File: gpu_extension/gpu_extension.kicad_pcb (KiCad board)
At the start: 4 copper layers, 70 x 50 mm, 89 parts, among them J1 Conn_02x10_Odd_Even, J2 DB15_Female_HighDensity_Mount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, J201 Conn_01x03_Male, J202 Conn_01x03_Male, J302 NOT_HDMI_A, Q1 BS170F, Q2 BS170F, Q3 BS170F, Q4 BS170F, U1 W25Q32JVSS, U2 IPS1604, U4 RP2040, U403 W25Q128JVS, U6 RP2040, Y201 ECS-120-8-36-CGN-TR, Y202 ECS-120-8-36-CGN-TR

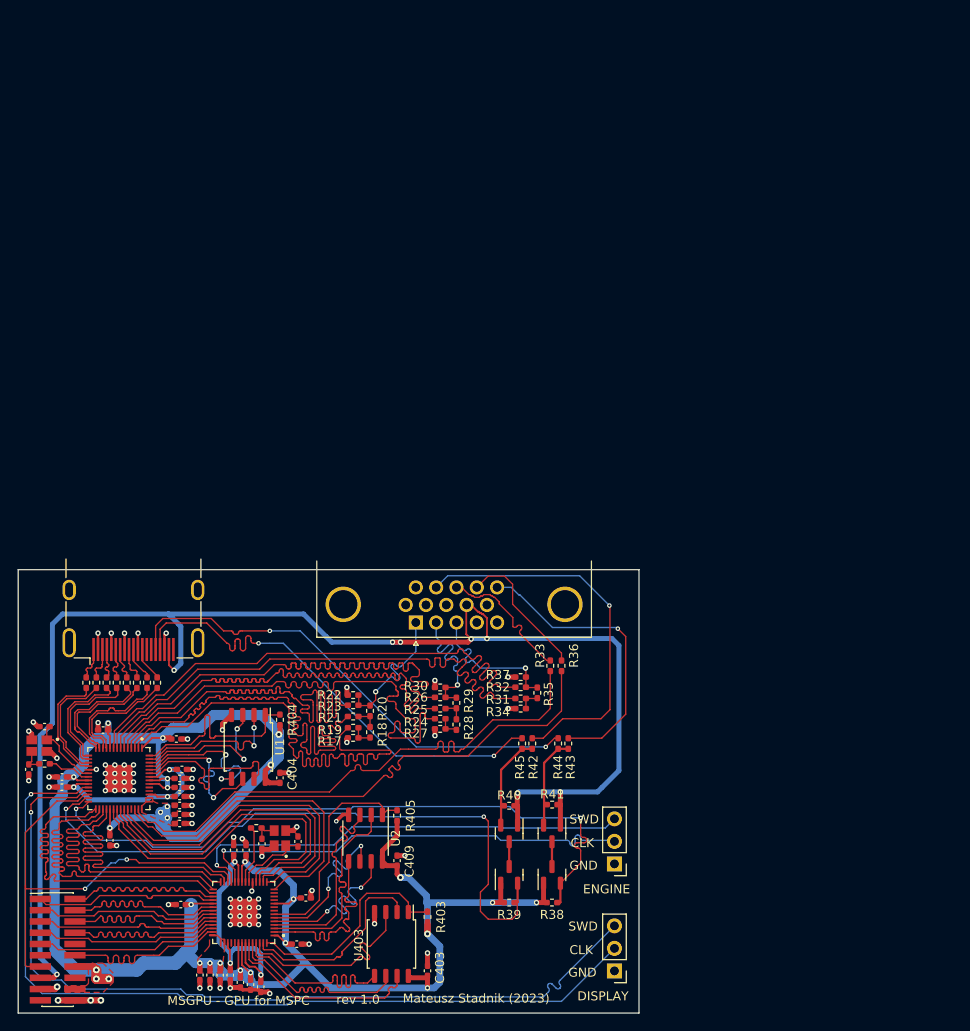
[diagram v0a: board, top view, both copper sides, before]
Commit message: prepared first versions of PCBs
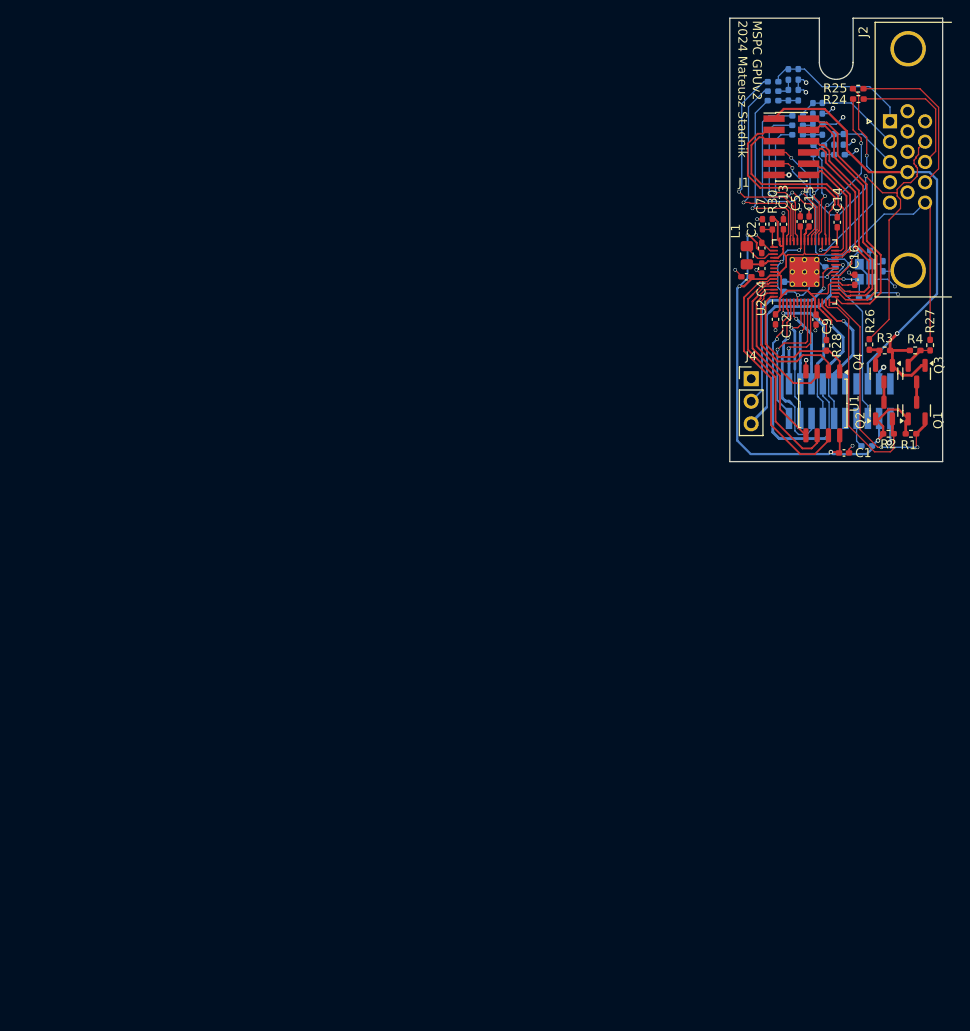
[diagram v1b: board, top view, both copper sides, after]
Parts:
- removed C201, C202, C218, C223: 14p, Capacitor_SMD:C_0402_1005Metric_Pad0.74x0.62mm_HandSolder
- removed C203, C204, C205, C206, C207, C209, C210, C211, C212, C213, C215, C216, C219, C220, C221, C222, C224, C225, C226, C227, C403, C404, C409: 100n, Capacitor_SMD:C_0402_1005Metric_Pad0.74x0.62mm_HandSolder
- removed C208, C214, C217, C228: 1u, Capacitor_SMD:C_0402_1005Metric_Pad0.74x0.62mm_HandSolder
- removed J201, J202: Conn_01x03_Male, Connector_PinHeader_2.54mm:PinHeader_1x03_P2.54mm_Vertical
- removed J302: NOT_HDMI_A, Connector_HDMI:HDMI_A_Molex_208658-1001_Horizontal
- removed R201, R202: 1k, Resistor_SMD:R_0402_1005Metric_Pad0.72x0.64mm_HandSolder
- removed R315, R316, R317, R318, R319, R320, R321, R322: 270, Resistor_SMD:R_0402_1005Metric_Pad0.72x0.64mm_HandSolder
- removed R32, R34: 536, Resistor_SMD:R_0402_1005Metric_Pad0.72x0.64mm_HandSolder
- removed R33, R36: 47, Resistor_SMD:R_0402_1005Metric_Pad0.72x0.64mm_HandSolder
- removed R35: 267, Resistor_SMD:R_0402_1005Metric_Pad0.72x0.64mm_HandSolder
- removed R37: 105, Resistor_SMD:R_0402_1005Metric_Pad0.72x0.64mm_HandSolder
- removed R38, R39, R40, R403, R404, R405, R41: 10k, Resistor_SMD:R_0402_1005Metric_Pad0.72x0.64mm_HandSolder
- removed R42, R43, R44, R45: 0, Resistor_SMD:R_0402_1005Metric_Pad0.72x0.64mm_HandSolder
- removed U4, U6: RP2040, footprints:QFN40P700X700X90-57N
- removed U403: W25Q128JVS, Package_SO:SOIC-8_5.23x5.23mm_P1.27mm
- removed Y201, Y202: ECS-120-8-36-CGN-TR, footprints:XTAL_ECS-120-8-36-CGN-TR
- added C1: 100n, Capacitor_SMD:C_0402_1005Metric_Pad0.74x0.62mm_HandSolder, F.Cu at (128.1, 116.8)
- added C10: 100n, Capacitor_SMD:C_0402_1005Metric_Pad0.74x0.62mm_HandSolder, F.Cu at (117.1, 97.0)
- added C11: 14p, Capacitor_SMD:C_0402_1005Metric_Pad0.74x0.62mm_HandSolder, B.Cu at (132.5, 95.8)
- added C12: 100n, Capacitor_SMD:C_0402_1005Metric_Pad0.74x0.62mm_HandSolder, F.Cu at (120.4, 101.8)
- added C13: 100n, Capacitor_SMD:C_0402_1005Metric_Pad0.74x0.62mm_HandSolder, F.Cu at (121.3, 91.1)
- added C14: 100n, Capacitor_SMD:C_0402_1005Metric_Pad0.74x0.62mm_HandSolder, F.Cu at (127.4, 90.8)
- added C15: 100n, Capacitor_SMD:C_0402_1005Metric_Pad0.74x0.62mm_HandSolder, F.Cu at (124.2, 90.7)
- added C16: 100n, Capacitor_SMD:C_0402_1005Metric_Pad0.74x0.62mm_HandSolder, F.Cu at (129.3, 97.3)
- added C2: 4.7u, Capacitor_SMD:C_0402_1005Metric_Pad0.74x0.62mm_HandSolder, F.Cu at (118.8, 93.7)
- added C3: 100n, Capacitor_SMD:C_0402_1005Metric_Pad0.74x0.62mm_HandSolder, B.Cu at (121.4, 98.1)
- added C4: 4.7u, Capacitor_SMD:C_0402_1005Metric_Pad0.74x0.62mm_HandSolder, F.Cu at (118.8, 96.0)
- added C5: 100n, Capacitor_SMD:C_0402_1005Metric_Pad0.74x0.62mm_HandSolder, F.Cu at (123.2, 90.7)
- added C6: 4.7u, Capacitor_SMD:C_0402_1005Metric_Pad0.74x0.62mm_HandSolder, B.Cu at (126.6, 95.9)
- added C7: 4.7u, Capacitor_SMD:C_0402_1005Metric_Pad0.74x0.62mm_HandSolder, F.Cu at (118.9, 91.1)
- added C8: 14p, Capacitor_SMD:C_0402_1005Metric_Pad0.74x0.62mm_HandSolder, B.Cu at (130.4, 99.3)
- added C9: 100n, Capacitor_SMD:C_0402_1005Metric_Pad0.74x0.62mm_HandSolder, F.Cu at (125.0, 101.8)
- added J3: Conn_02x10_Odd_Even, Connector_PinHeader_1.27mm:PinHeader_2x10_P1.27mm_Vertical_SMD, B.Cu at (127.6, 111.0)
- added J4: Conn_01x03_Male, Connector_PinHeader_2.54mm:PinHeader_1x03_P2.54mm_Vertical, F.Cu at (117.7, 108.5)
- added L1: 3.3u, Inductor_SMD:L_0805_2012Metric_Pad1.15x1.40mm_HandSolder, F.Cu at (117.2, 94.5)
- added R1: 10k, Resistor_SMD:R_0402_1005Metric_Pad0.72x0.64mm_HandSolder, F.Cu at (135.7, 114.7)
- added R10: 619, Resistor_SMD:R_0402_1005Metric_Pad0.72x0.64mm_HandSolder, B.Cu at (120.1, 77.1)
- added R11: 619, Resistor_SMD:R_0402_1005Metric_Pad0.72x0.64mm_HandSolder, B.Cu at (120.1, 76.0)
- added R12: 619, Resistor_SMD:R_0402_1005Metric_Pad0.72x0.64mm_HandSolder, B.Cu at (120.1, 75.0)
- added R13: 536, Resistor_SMD:R_0402_1005Metric_Pad0.72x0.64mm_HandSolder, B.Cu at (127.6, 83.2)
- added R14: 267, Resistor_SMD:R_0402_1005Metric_Pad0.72x0.64mm_HandSolder, B.Cu at (127.0, 81.5)
- added R15: 105, Resistor_SMD:R_0402_1005Metric_Pad0.72x0.64mm_HandSolder, B.Cu at (128.1, 81.5)
- added R16: 619, Resistor_SMD:R_0402_1005Metric_Pad0.72x0.64mm_HandSolder, B.Cu at (125.7, 80.4)
- added R2: 10k, Resistor_SMD:R_0402_1005Metric_Pad0.72x0.64mm_HandSolder, F.Cu at (133.1, 114.7)
- added R3: 10k, Resistor_SMD:R_0402_1005Metric_Pad0.72x0.64mm_HandSolder, F.Cu at (132.7, 105.3)
- added R4: 10k, Resistor_SMD:R_0402_1005Metric_Pad0.72x0.64mm_HandSolder, F.Cu at (136.1, 105.3)
- added R5: 536, Resistor_SMD:R_0402_1005Metric_Pad0.72x0.64mm_HandSolder, B.Cu at (125.3, 83.2)
- added R6: 536, Resistor_SMD:R_0402_1005Metric_Pad0.72x0.64mm_HandSolder, B.Cu at (125.3, 82.1)
- added R7: 619, Resistor_SMD:R_0402_1005Metric_Pad0.72x0.64mm_HandSolder, B.Cu at (122.9, 81.0)
- added R8: 619, Resistor_SMD:R_0402_1005Metric_Pad0.72x0.64mm_HandSolder, B.Cu at (122.9, 79.9)
- added R9: 619, Resistor_SMD:R_0402_1005Metric_Pad0.72x0.64mm_HandSolder, B.Cu at (122.9, 78.8)
- added Y1: ECS-120-8-36-CGN-TR, footprints:XTAL_ECS-120-8-36-CGN-TR, B.Cu at (130.5, 96.4)
- J1: value Conn_02x10_Odd_Even -> Conn_02x06_Odd_Even; footprint Connector_PinHeader_1.27mm:PinHeader_2x10_P1.27mm_Vertical_SMD -> Connector_PinHeader_1.27mm:PinHeader_2x06_P1.27mm_Vertical_SMD
- R17, R21: value 619 -> 309; moved to B.Cu
- R18: moved to B.Cu
- R19, R23: value 619 -> 97.6; moved to B.Cu
- R20: value 309 -> 619; moved to B.Cu
- R22: value 97.6 -> 309; moved to B.Cu
- R24, R25: value 619 -> 47
- R26, R27: value 619 -> 0
- R28: value 309 -> 10k
- R29: value 309 -> < 10k; moved to B.Cu
- R30: value 97.6 -> 33
- R31: value 536 -> 1k; moved to B.Cu
- U2: value IPS1604 -> RP2350_60QFN; footprint Package_SO:SOP-8_3.9x4.9mm_P1.27mm -> RP2350_60QFN_minimal:RP2350-QFN-60-1EP_7x7_P0.4mm_EP3.4x3.4mm_ThermalVias
- moved J1 122.6 mm to (122.2, 82.3)
- moved R19 87.6 mm to (125.7, 78.0), turned to -90 degrees
- moved R23 87.1 mm to (123.0, 74.2), turned to -90 degrees
- moved R18 86.3 mm to (124.6, 78.0)
- moved R17 86.0 mm to (124.6, 80.4), turned to 90 degrees
- moved R21 85.5 mm to (121.8, 76.5), turned to 90 degrees
- moved R22 85.5 mm to (121.8, 74.2), turned to 90 degrees
- moved R20 84.6 mm to (123.0, 76.5), turned to -90 degrees
- moved R25 84.3 mm to (129.7, 75.8), turned to 180 degrees
- moved R24 84.3 mm to (129.7, 76.9), turned to 180 degrees
- moved U2 80.8 mm to (123.7, 96.4), turned to 90 degrees
- moved J2 77.8 mm to (133.3, 79.5), turned to 90 degrees
- moved U1 75.5 mm to (125.7, 111.3)
- moved R27 70.2 mm to (137.8, 104.7), turned to -90 degrees
- moved Q3 69.9 mm to (136.3, 107.9), turned to -90 degrees
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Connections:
- J1 pad 1: /Render Engine/BUS connector/BUS.D6 -> +5V
- J1 pad 10: unconnected-(J1-Pin_10) -> /DVI connector/DVI.D2+
- J1 pad 11: unconnected-(J1-Pin_11) -> GND
- J1 pad 12: /Render Engine/BUS connector/BUS.CS# -> /DVI connector/DVI.D2-
- J1 pad 2: /Render Engine/BUS connector/BUS.D7 -> /DVI connector/DVI.D0+
- J1 pad 3: /Render Engine/BUS connector/BUS.D4 -> /DVI connector/DVI.CK-
- J1 pad 4: /Render Engine/BUS connector/BUS.D5 -> /DVI connector/DVI.D0-
- J1 pad 5: /Render Engine/BUS connector/BUS.D2 -> /DVI connector/DVI.CK+
- J1 pad 6: /Render Engine/BUS connector/BUS.D3 -> /DVI connector/DVI.D1+
- J1 pad 7: /Render Engine/BUS connector/BUS.D0 -> /DVI connector/CEC_I2C_DATA
- J1 pad 8: /Render Engine/BUS connector/BUS.D1 -> /DVI connector/DVI.D1-
- J1 pad 9: /Render Engine/BUS connector/BUS.CLK -> /DVI connector/CEC_I2C_CLOCK
- J2 pad 12: Net-(J2-Pad12) -> /DVI connector/CEC_I2C_DATA
- J2 pad 15: Net-(J2-Pad15) -> /DVI connector/CEC_I2C_CLOCK
- Q1 pad 2: /DVI connector/MCU_I2C.DATA -> /DVI connector/MCU_I2C.CLOCK
- Q2 pad 1: +5V -> +3V3
- Q2 pad 2: /DVI connector/CEC_I2C_DATA -> /DVI connector/MCU_I2C.DATA
- Q2 pad 3: Net-(Q1-D) -> Net-(Q2-D)
- Q3 pad 1: +3V3 -> +5V
- Q3 pad 2: /DVI connector/MCU_I2C.CLOCK -> Net-(Q3-S)
- Q3 pad 3: Net-(Q3-D) -> Net-(Q1-D)
- Q4 pad 2: /DVI connector/CEC_I2C_CLOCK -> Net-(Q4-S)
- Q4 pad 3: Net-(Q3-D) -> Net-(Q2-D)
- R17 pad 1: GND -> Net-(R16-Pad2)
- R18 pad 2: Net-(R18-Pad2) -> /DVI connector/VGA_G
- R19 pad 1: /DVI connector/VGA.R0 -> /DVI connector/VGA_G
- R19 pad 2: Net-(R17-Pad2) -> GND
- R20 pad 1: Net-(R18-Pad2) -> GND
- R20 pad 2: /DVI connector/VGA_R -> Net-(R10-Pad2)
- R21 pad 1: /DVI connector/VGA.R1 -> Net-(R10-Pad2)
- R21 pad 2: Net-(R18-Pad2) -> Net-(R11-Pad2)
- R22 pad 1: /DVI connector/VGA_R -> Net-(R11-Pad2)
- R22 pad 2: GND -> /DVI connector/VGA_R
- R23 pad 1: /DVI connector/VGA.R2 -> /DVI connector/VGA_R
- R23 pad 2: /DVI connector/VGA_R -> GND
- R24 pad 1: /DVI connector/VGA.G0 -> /DVI connector/VGA_HSYNC
- R24 pad 2: Net-(R24-Pad2) -> /DVI connector/VGA.HSYNC
- R25 pad 1: /DVI connector/VGA.G1 -> /DVI connector/VGA_VSYNC
- R25 pad 2: Net-(R25-Pad2) -> /DVI connector/VGA.VSYNC
- R26 pad 1: /DVI connector/VGA.G2 -> /DVI connector/CEC_I2C_DATA
- R26 pad 2: /DVI connector/VGA_G -> Net-(Q4-S)
- R27 pad 1: GND -> /DVI connector/CEC_I2C_CLOCK
- R27 pad 2: Net-(R24-Pad2) -> Net-(Q3-S)
- R28 pad 1: Net-(R24-Pad2) -> +3V3
- R28 pad 2: Net-(R25-Pad2) -> /Memory/QSPI.CS#
- R29 pad 1: Net-(R25-Pad2) -> +3V3
- R29 pad 2: /DVI connector/VGA_G -> /BUS connector/BUS.DET#
- R30 pad 1: /DVI connector/VGA_G -> +3V3
- R30 pad 2: GND -> /VREG_AVDD
- R31 pad 1: /DVI connector/VGA.B0 -> Net-(Y1-OUT/IN)
- R31 pad 2: Net-(R31-Pad2) -> /OSC_OUT
- U1 pad 1: /Memory/FLASH.CS# -> /Memory/QSPI.CS#
- U1 pad 2: /Memory/FLASH.IO1 -> /Memory/QSPI.IO1
- U1 pad 3: /Memory/FLASH.IO2 -> /Memory/QSPI.IO2
- U1 pad 5: /Memory/FLASH.IO0 -> /Memory/QSPI.IO0
- U1 pad 6: /Memory/FLASH.CLK -> /Memory/QSPI.CLK
- U1 pad 7: /Memory/FLASH.IO3 -> /Memory/QSPI.IO3
- U2 pad 1: /Render Engine/Memory Render Engine/PSRAM.CE# -> +3V3
- U2 pad 2: /Render Engine/Memory Render Engine/PSRAM.IO1 -> /BUS connector/BUS.D0
- U2 pad 3: /Render Engine/Memory Render Engine/PSRAM.IO2 -> /BUS connector/BUS.D1
- U2 pad 4: GND -> /BUS connector/BUS.D2
- U2 pad 5: /Render Engine/Memory Render Engine/PSRAM.IO0 -> /BUS connector/BUS.D3
- U2 pad 6: /Render Engine/Memory Render Engine/PSRAM.CLK -> +1V1
- U2 pad 7: /Render Engine/Memory Render Engine/PSRAM.IO3 -> /BUS connector/BUS.D4
- U2 pad 8: +3V3 -> /BUS connector/BUS.D5
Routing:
- net +3V3: track 295.3 -> 107.8 mm, vias 28 -> 4
- net +5V: track 163.1 -> 60.6 mm, vias 8 -> 1
- net /DEBUG.SWCLK: track 98.0 -> 22.2 mm
- net /DEBUG.SWD: track 97.9 -> 26.0 mm
- net Net-(J302-SCL): track 55.2 -> 0.00 mm, vias 2 -> 0
- net Net-(J302-SDA): track 55.1 -> 0.00 mm, vias 2 -> 0
- net /Render Engine/BUS connector/BUS.RE#: track 51.7 -> 0.00 mm, vias 2 -> 0
- net /DVI connector/VGA.B0: track 62.1 -> 10.6 mm, vias 0 -> 1
- net /Render Engine/DEBUG.SWD: track 51.2 -> 0.00 mm, vias 1 -> 0
- net /Render Engine/DEBUG.SWCLK: track 50.8 -> 0.00 mm, vias 1 -> 0
- net /DVI connector/VGA.B1: track 62.1 -> 11.7 mm, vias 0 -> 1
- net /DVI connector/MCU_I2C.DATA: track 74.3 -> 25.5 mm, vias 2 -> 0
- net /DVI connector/MCU_I2C.CLOCK: track 75.8 -> 27.2 mm
- net /BUS connector/BUS.D1: track 0.00 -> 46.8 mm, vias 0 -> 1
- net /DVI connector/VGA.G0: track 61.9 -> 15.2 mm, vias 0 -> 1
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- removed copper zone on F.Cu, net +3V3
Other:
- board size 70 x 50 mm -> 24 x 50 mm
- board text added: "MSPC GPUv2 2024 Mateusz Stadnik"
- board text removed: "CLK"
- board text removed: "DISPLAY"
- board text removed: "ENGINE"
- board text removed: "GND"
- board text removed: "MSGPU - GPU for MSPC"
- board text removed: "Mateusz Stadnik (2023)"
- board text removed: "SWD"
- board text removed: "rev 1.0"
